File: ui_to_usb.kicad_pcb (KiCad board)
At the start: 4 copper layers, 39.2 x 29 mm, 43 parts, among them J1 TYPE-C-31-M-12, J2 PM254-2-06-S-8.5, J3 BM12B-SRSS-TB, SW1 TS24CA, SW2 TS24CA, U1 SPX3819M5-L, U2 USBLC6-2SC6, U3 CH32V203K8T6, Y1 8M

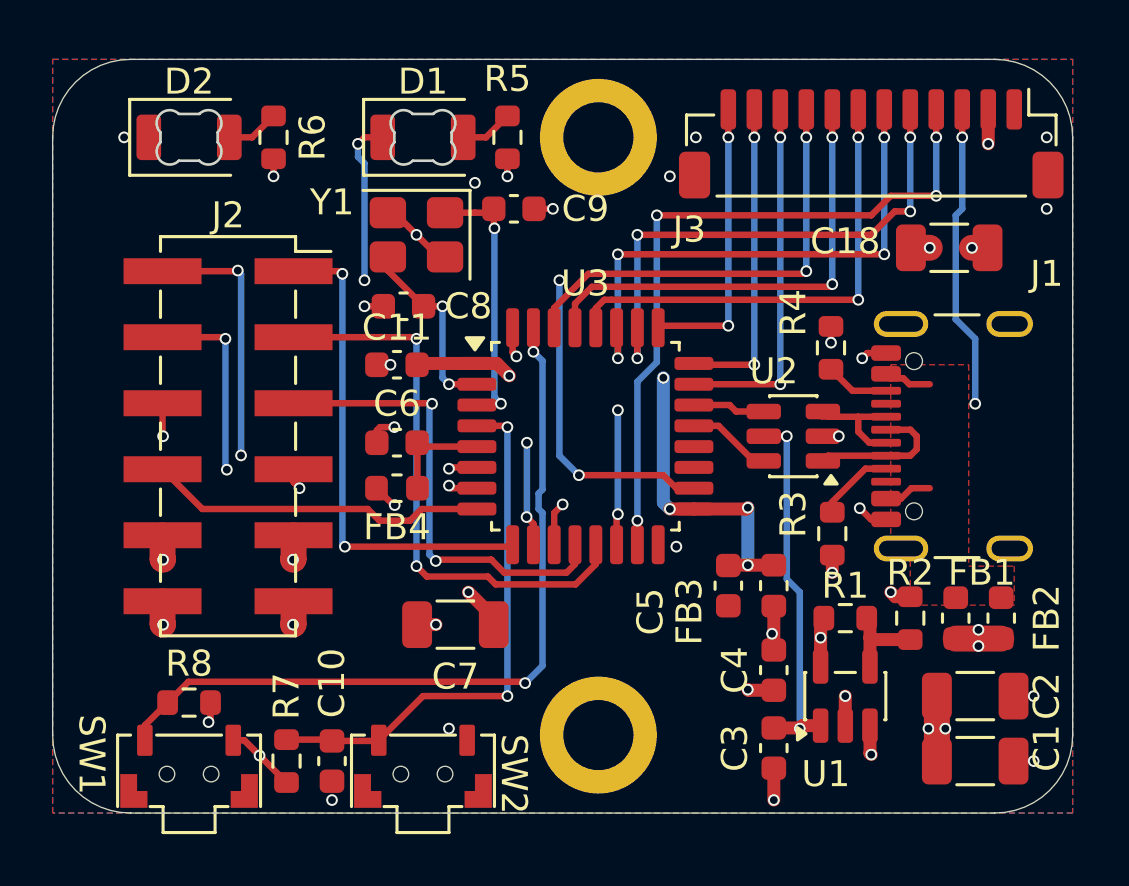
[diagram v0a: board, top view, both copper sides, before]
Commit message: Layout looks decent. Ready to order.
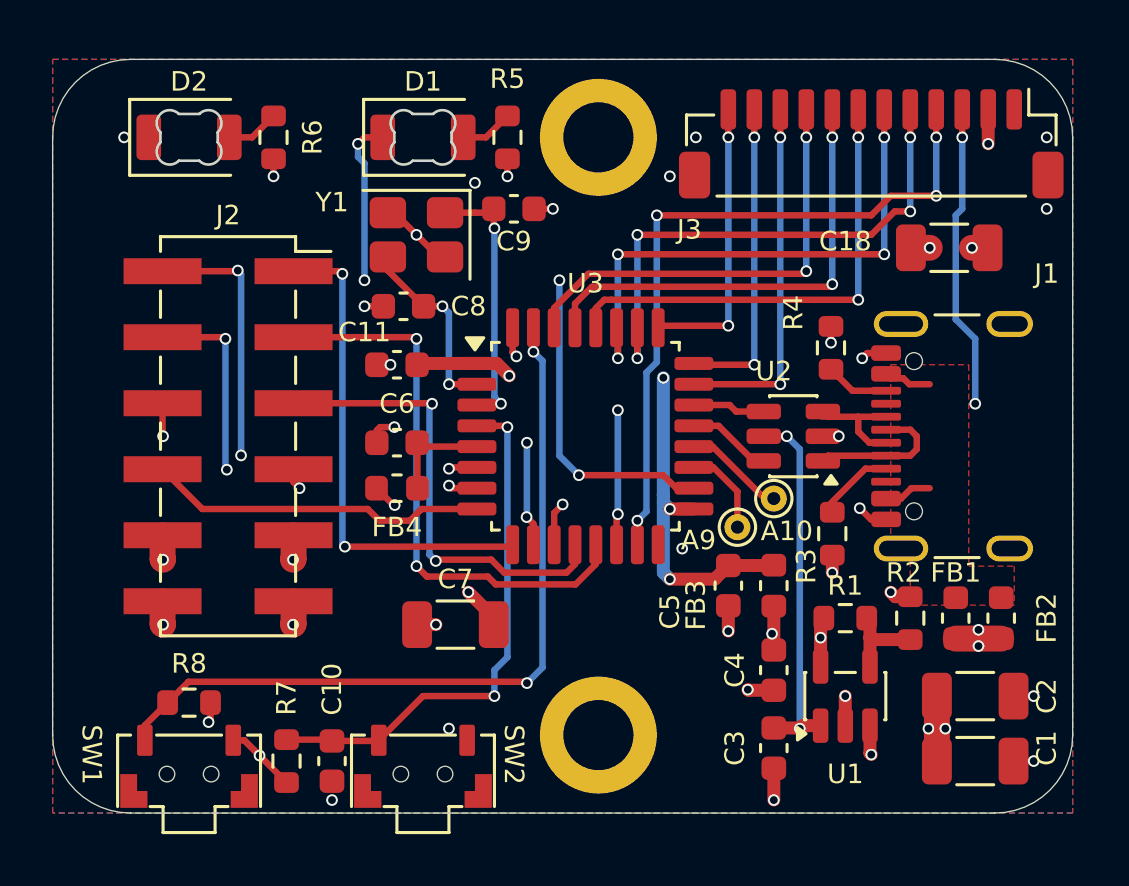
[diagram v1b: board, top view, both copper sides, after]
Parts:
- removed the G*** at (85.2, 88.4)
- removed the G*** at (92.3, 75.6)
- added A10: U_RX, TestPoint:TestPoint_Pad_D1.0mm, F.Cu at (102.0, 82.4)
- added A9: U_TX, TestPoint:TestPoint_Pad_D1.0mm, F.Cu at (100.6, 83.5)
- added G***: LOGO, LOGO, B.Cu at (93.6, 73.1)
- added G***: LOGO, LOGO, B.Cu at (82.5, 86.3)
- moved G1 14.5 mm to (108.3, 80.0)
- moved G2 8.55 mm to (94.5, 83.4)
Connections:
- U3 pad 19: unconnected-(U3-PA9-Pad19) -> Net-(U3-PA9)
- U3 pad 20: unconnected-(U3-PA10-Pad20) -> Net-(U3-PA10)
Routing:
- net Net-(U3-PA10): track 0.00 -> 3.90 mm
- net Net-(U3-PA9): track 0.00 -> 3.43 mm
- net VDD: track 21.9 -> 23.4 mm, vias 5 -> 4
- net GND: track 20.6 -> 21.6 mm, vias 31 -> 32
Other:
- board text added: "A10"
- board text added: "A9"
- board text added: "B"
- board text added: "R"
- board text added: "betz-engineering.ch/open_hardware/ui_to_usb/"
- board text removed: "https://github.com/betz-engineering/ui_to_usb"
